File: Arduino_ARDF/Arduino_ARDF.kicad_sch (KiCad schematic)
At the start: 37 parts, among them J1 Output Mode, J2 Programming, J3 Analog 2, J4 AUX2, J5 Analog 1, J7 Analog 0, J8 AUX1, SW1 Button 1, SW2 Button 2, U1 ATmega328-P, U20 L78L05_TO92, Y1 16M

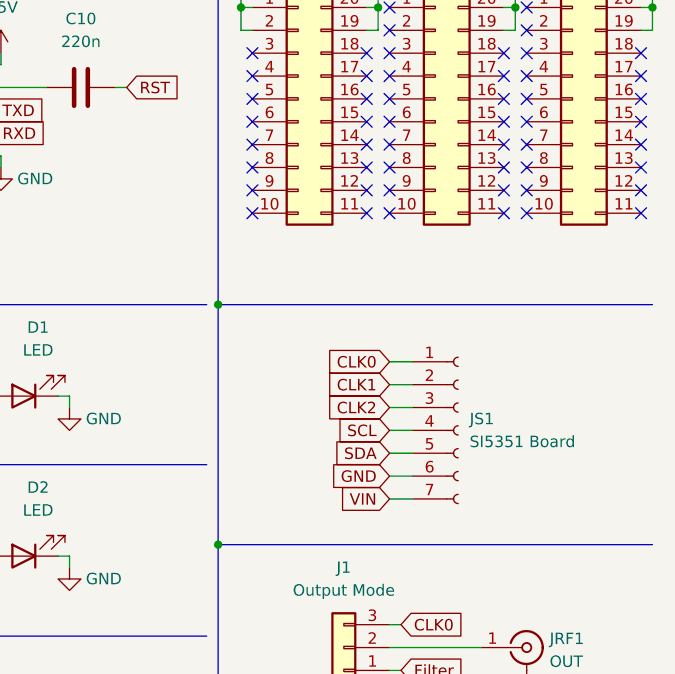
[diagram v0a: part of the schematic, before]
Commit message: Ricominciato PCB
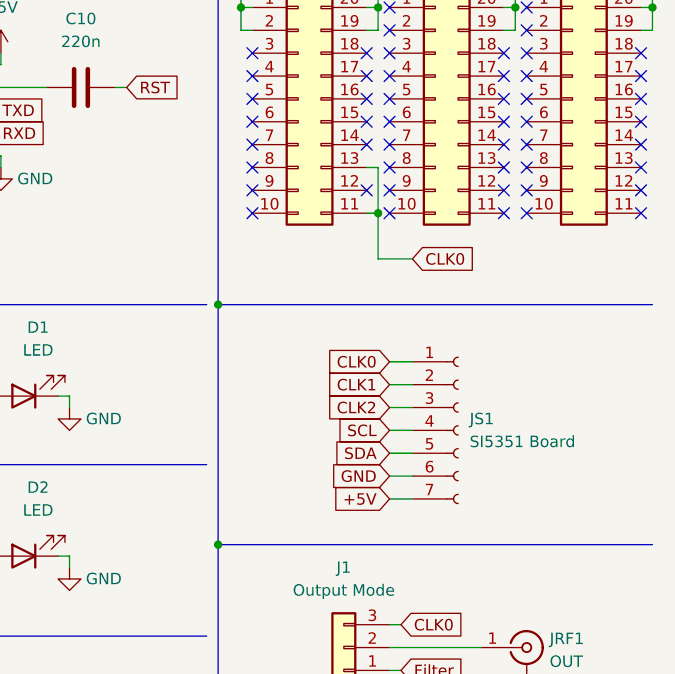
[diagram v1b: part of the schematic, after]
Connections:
- net +5V: now also JS1.7 (Pin_7)
- net CLK0: now also JF3.11 (Pin_11), JF3.13 (Pin_13)
- net VIN: no longer JS1.7 (Pin_7)
- no-connect marks 57 -> 55
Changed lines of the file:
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@@
   (junction (at 44.45 83.82) (diameter 0) (color 0 0 0 0)
+  )
+  (junction (at 252.73 49.53) (diameter 0) (color 0 0 0 0)
   )
   (junction (at 162.56 54.61) (diameter 0) (color 0 0 0 0)
@@
   (no_connect (at 238.76 36.83))
   (no_connect (at 254 34.29))
-  (no_connect (at 251.46 49.53))
   (no_connect (at 254 49.53))
   (no_connect (at 266.7 49.53))
@@
   (no_connect (at 254 41.91))
   (no_connect (at 266.7 39.37))
-  (no_connect (at 251.46 44.45))
   (no_connect (at 57.15 71.12))
   (no_connect (at 57.15 73.66))
@@
     (stroke (width 0) (type default) (color 0 0 0 0))
   )
+  (wire (pts (xy 252.73 44.45) (xy 252.73 49.53))
+    (stroke (width 0) (type default) (color 0 0 0 0))
+  )
   (bus (pts (xy 182.88 119.38) (xy 182.88 142.24))
     (stroke (width 0) (type default) (color 0 0 0 0))
@@
     (stroke (width 0) (type default) (color 0 0 0 0))
   )
+  (wire (pts (xy 252.73 54.61) (xy 256.54 54.61))
+    (stroke (width 0) (type default) (color 0 0 0 0))
+  )
   (wire (pts (xy 172.72 59.69) (xy 176.53 59.69))
     (stroke (width 0) (type default) (color 0 0 0 0))
@@
     (stroke (width 0) (type default) (color 0 0 0 0))
   )
+  (wire (pts (xy 252.73 49.53) (xy 252.73 54.61))
+    (stroke (width 0) (type default) (color 0 0 0 0))
+  )
   (wire (pts (xy 267.97 15.24) (xy 256.54 15.24))
     (stroke (width 0) (type default) (color 0 0 0 0))
@@
     (stroke (width 0) (type default) (color 0 0 0 0))
   )
+  (wire (pts (xy 251.46 49.53) (xy 252.73 49.53))
+    (stroke (width 0) (type default) (color 0 0 0 0))
+  )
   (wire (pts (xy 198.12 128.27) (xy 195.58 128.27))
     (stroke (width 0) (type default) (color 0 0 0 0))
@@
   )
   (wire (pts (xy 208.28 33.02) (xy 210.82 33.02))
+    (stroke (width 0) (type default) (color 0 0 0 0))
+  )
+  (wire (pts (xy 251.46 44.45) (xy 252.73 44.45))
     (stroke (width 0) (type default) (color 0 0 0 0))
   )
@@
     )
   )
+  (global_label "CLK0" (shape input) (at 256.54 54.61 0) (fields_autoplaced)
+    (effects (font (size 1.27 1.27)) (justify left))
+    (property "Intersheet References" "${INTERSHEET_REFS}" (id 0) (at 263.7307 54.6894 0)
+      (effects (font (size 1.27 1.27)) (justify left) hide)
+    )
+  )
   (global_label "SCL" (shape input) (at 58.42 66.04 0) (fields_autoplaced)
     (effects (font (size 1.27 1.27)) (justify left))
@@
     )
   )
-  (global_label "VIN" (shape input) (at 254 81.28 180) (fields_autoplaced)
-    (effects (font (size 1.27 1.27)) (justify right))
-    (property "Intersheet References" "${INTERSHEET_REFS}" (id 0) (at 248.5631 81.2006 0)
-      (effects (font (size 1.27 1.27)) (justify right) hide)
-    )
+  (global_label "+5V" (shape input) (at 254 81.28 180) (fields_autoplaced)
+    (effects (font (size 1.27 1.27)) (justify right))
+    (property "Intersheet References" "${INTERSHEET_REFS}" (id 0) (at 247.7164 81.2006 0)
+      (effects (font (size 1.27 1.27)) (justify right) hide)
+    )
